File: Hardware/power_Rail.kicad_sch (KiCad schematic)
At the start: 2 parts

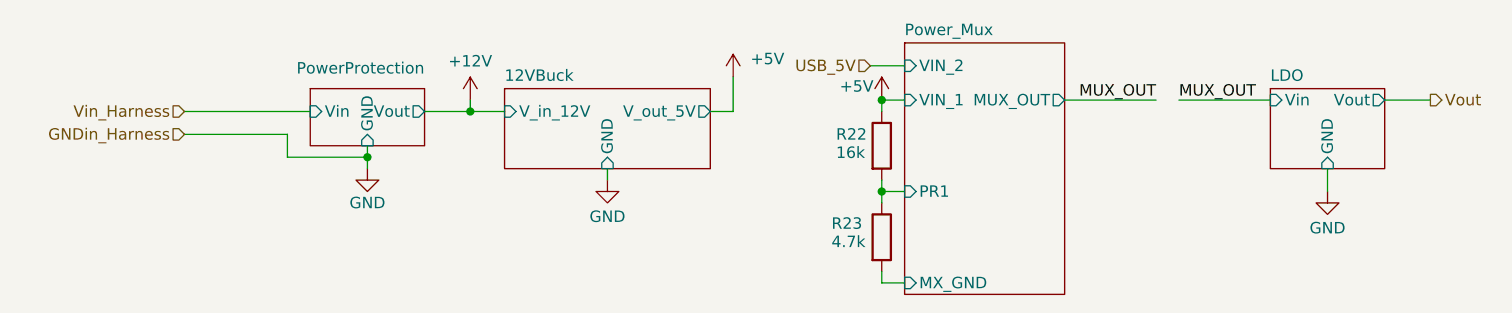
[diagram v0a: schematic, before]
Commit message: fixed some subsheets
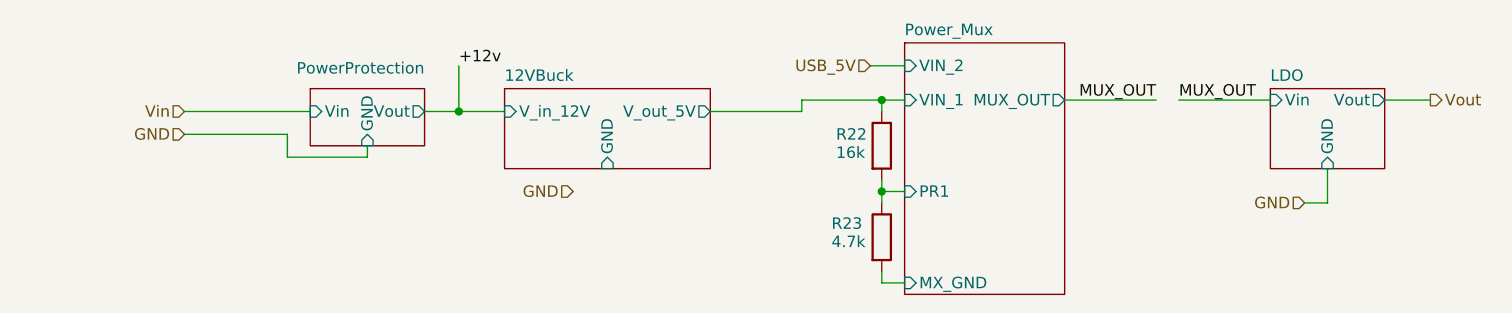
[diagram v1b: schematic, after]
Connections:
- net +5V renamed 12VBuck/V_out_5V
